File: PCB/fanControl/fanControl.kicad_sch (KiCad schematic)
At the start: 99 parts, among them J1 USB_B_Micro, J2 Barrel_Jack_Switch, J3 Conn_01x03, J4 Conn_01x06, J5 Conn_01x04, Q1 FDD4243, Q2 BSS84, Q3 BC547, Q4 BC847B, Q5 BC847B, Q6 BRCS4484, Q7 BC847B, Q8 BSS84, Q9 BC847B, U1 DS18B20, U2 CH340B, U3 LM2575BT-ADJ, U4 LM1117, U5 ESP-12E, Y1 12M

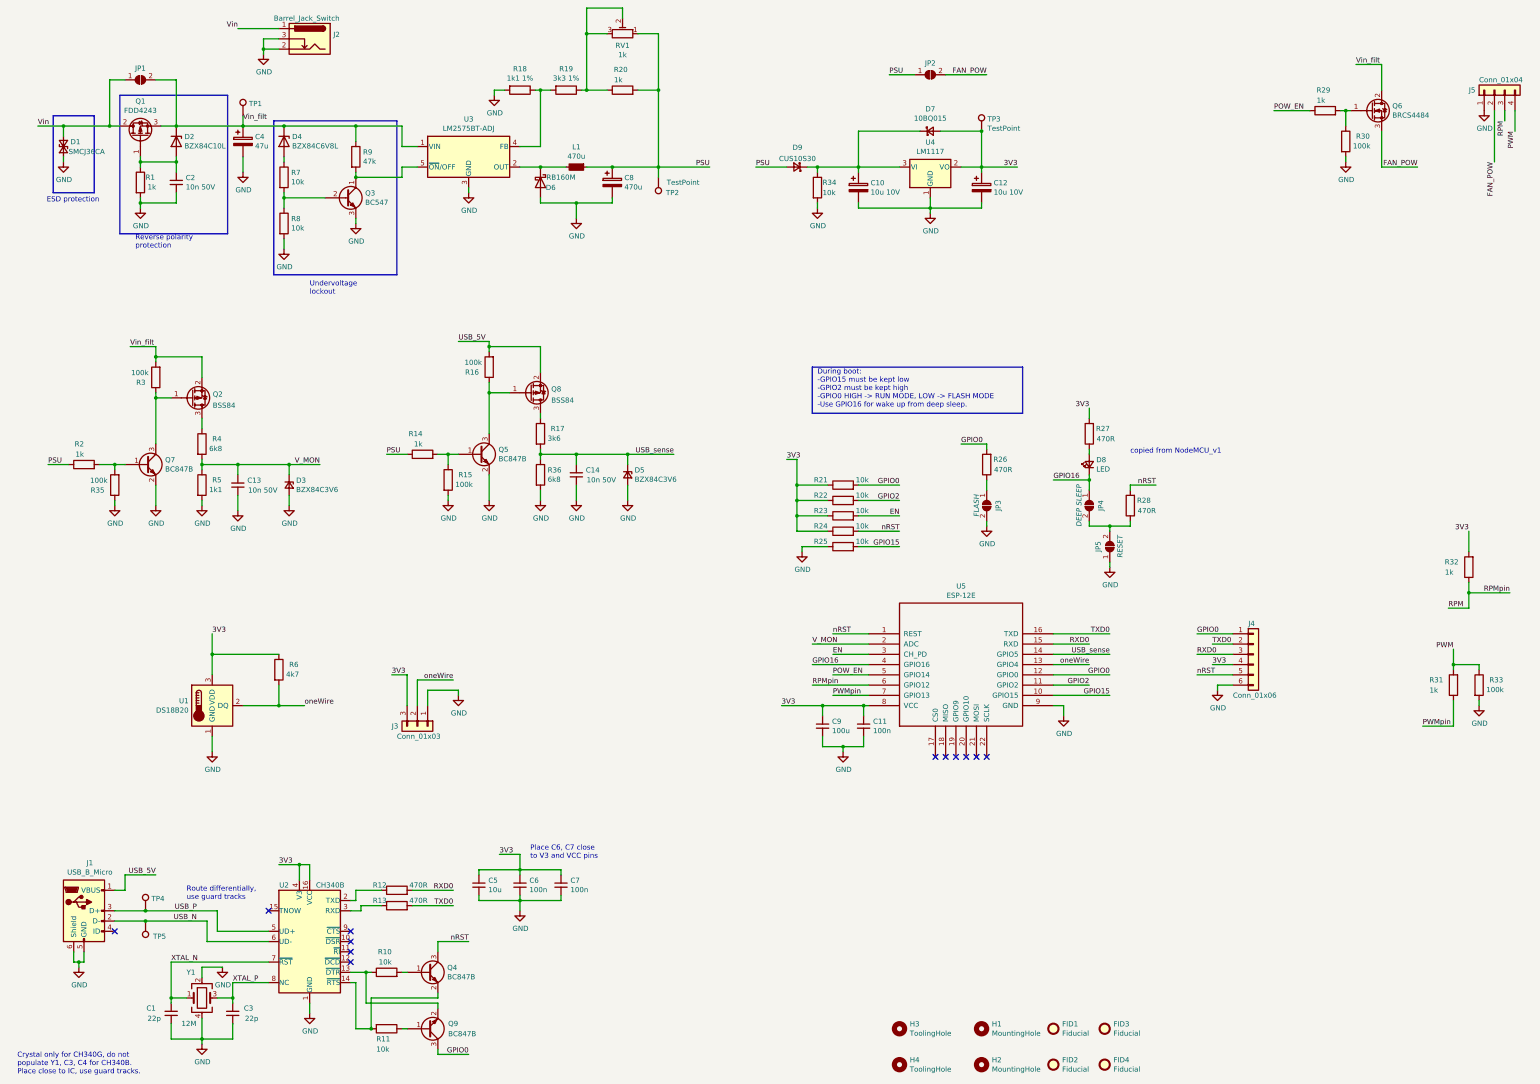
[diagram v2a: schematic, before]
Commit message: before optocouplers
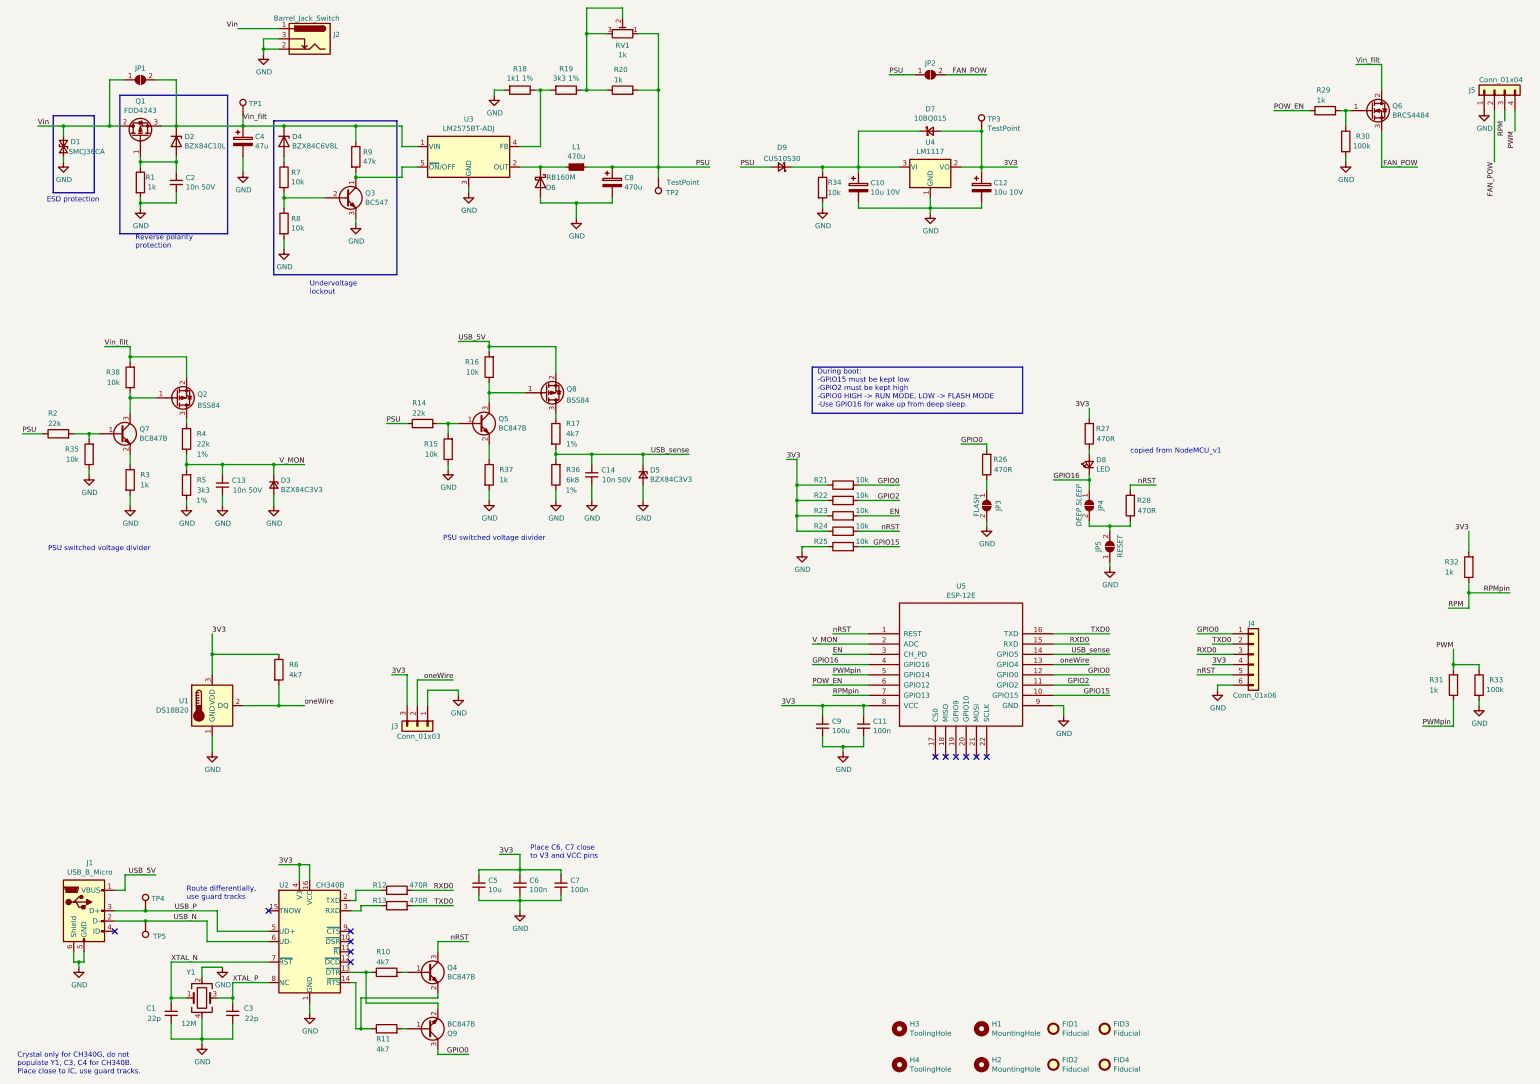
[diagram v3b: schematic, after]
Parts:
- added R37: 1k, agro-footprint:RES_0805, symbol Device:R
- added R38: 10k, agro-footprint:RES_0805, symbol Device:R
- D3, D5: value BZX84C3V6 -> BZX84C3V3; LCSC C94413 -> C82473; MPN BZX84C3V6LT1G -> BZX84C3V3LT1G
- D9, Q2, Q8: Supplier (none) -> LCSC
- R10, R11: value 10k -> 4k7; LCSC C100047 -> C60816; MPN RC0805JR-0710KL -> RC0805FR-074K7L; RMK (none) -> 1%
- R14, R2: value 1k -> 22k; LCSC C100046 -> C114565; MPN RC0805JR-071KL -> RC0805FR-0722KL; RMK (none) -> 1%
- R15, R16, R35: value 100k -> 10k; LCSC C100049 -> C100047; MPN RC0805JR-07100KL -> RC0805JR-0710KL
- R17: value 3k6 -> 4k7; LCSC C229201 -> C60816; MPN AC0805JR-073K6L -> RC0805FR-074K7L; RMK (none) -> 1%
- R3: value 100k -> 1k; LCSC C100049 -> C100046; MPN RC0805JR-07100KL -> RC0805JR-071KL
- R36: LCSC C137409 -> C114550; MPN RC0805JR-076K8L -> RC0805FR-076K8L; RMK (none) -> 1%
- R4: value 6k8 -> 22k; LCSC (none) -> C114565; MPN (none) -> RC0805FR-0722KL; RMK (none) -> 1%
- R5: value 1k1 -> 3k3; LCSC (none) -> C114531; MPN (none) -> RC0805FR-073K3L; RMK (none) -> 1%
- R6: LCSC C105427 -> C60816; MPN RC0805JR-074K7L -> RC0805FR-074K7L; RMK (none) -> 1%
- U5: footprint kicad-ESP8266:ESP-12E -> ESP8266:ESP-12E
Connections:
- net GND: now also R15.1, R3.2, R36.1, R5.1, R37.2; no longer Q5.2 (E), Q7.2 (E), R15.2, R36.2, R5.2
- net POW_EN: now also U5.6 (GPIO12); no longer U5.5 (GPIO14)
- net PWMpin: now also U5.5 (GPIO14); no longer U5.7 (GPIO13)
- net RPM: now also U5.7 (GPIO13); no longer U5.6 (GPIO12)
- net USB_sense: now also R36.2; no longer R36.1
- net V_MON: now also R5.2; no longer R5.1
- net Vin_filt: now also R38.2; no longer R3.2
- net at Q4.2 (E), U2.14 (~{RTS}): now also R11.1; no longer R11.2
- net at Q5.1 (B), R14.2: now also R15.2; no longer R15.1
- net at Q2.1 (G), Q7.3 (C): now also R38.1; no longer R3.1
- net at Q9.1 (B): now also R11.2; no longer R11.1
- new net: Q7.2 (E), R3.1
- new net: Q5.2 (E), R37.1
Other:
- note added: "PSU switched voltage divider"
- moved on the sheet: C13, C14, D3, D5, D9, Q2, Q5, Q7, Q8, R34

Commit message: RFQ2
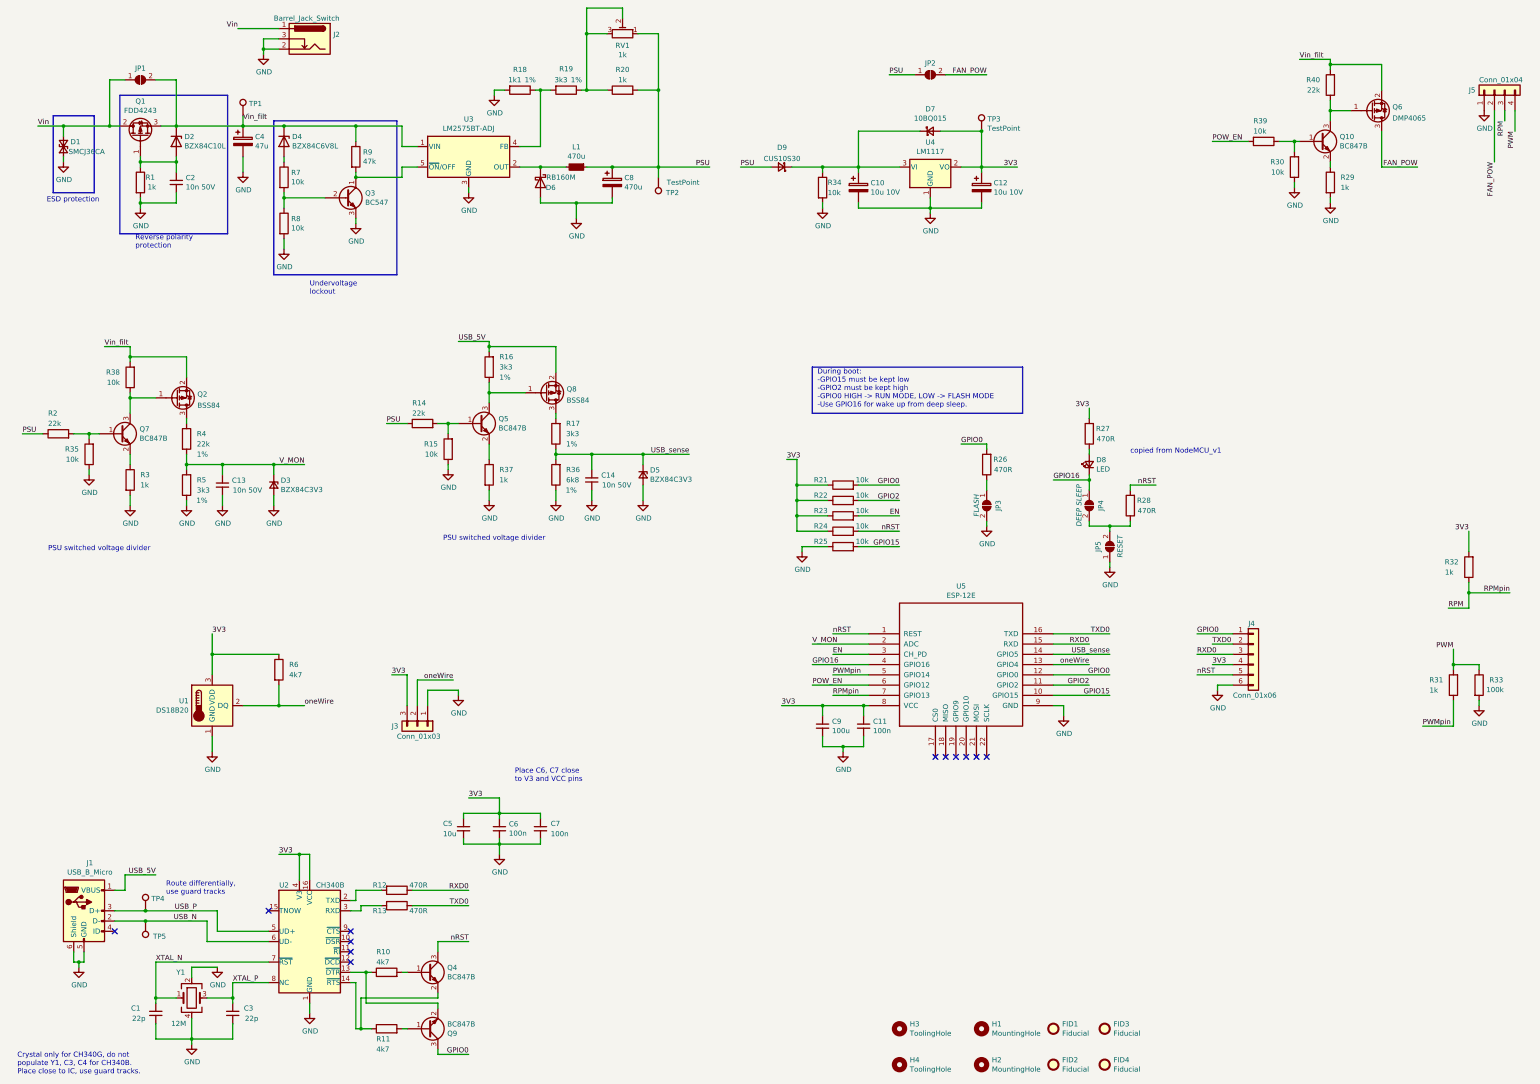
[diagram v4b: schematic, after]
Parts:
- removed Q6: BRCS4484, fanControl:BRCS4484, symbol Transistor_FET:IRF540N
- added Q10: BC847B, Package_TO_SOT_SMD:SOT-23, symbol Transistor_BJT:BC847
- added Q6: DMP4065, Package_TO_SOT_SMD:SOT-23, symbol Device:Q_PMOS_GSD
- added R39: 10k, agro-footprint:RES_0805, symbol Device:R
- added R40: 22k, agro-footprint:RES_0805, symbol Device:R
- R16: value 10k -> 3k3; LCSC C100047 -> C114531; MPN RC0805JR-0710KL -> RC0805FR-073K3L; RMK (none) -> 1%
- R17: value 4k7 -> 3k3; LCSC C60816 -> C114531; MPN RC0805FR-074K7L -> RC0805FR-073K3L
- R18: value 1k1 1% -> 1k1; RMK (none) -> 1%
- R19: value 3k3 1% -> 3k3; RMK (none) -> 1%
- R30: value 100k -> 10k; LCSC C100049 -> C100047; MPN RC0805JR-07100KL -> RC0805JR-0710KL
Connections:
- net FAN_POW: now also Q6.3 (D)
- net GND: now also R29.2, R30.1; no longer R30.2
- net POW_EN: now also R39.2; no longer R29.1
- net RXD0: now also R12.1; no longer R12.2
- net TXD0: now also R13.1; no longer R13.2
- net USB_sense: now also R17.1; no longer R17.2
- net Vin_filt: now also Q6.2 (S), R40.2
- net at U2.2 (TXD): now also R12.2; no longer R12.1
- net at U2.3 (RXD): now also R13.2; no longer R13.1
- net at Q8.3 (D): now also R17.2; no longer R17.1
- new net: Q10.3 (C), Q6.1 (G), R40.1
- new net: Q10.1 (B), R30.2, R39.1
- new net: Q10.2 (E), R29.1
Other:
- moved on the sheet: C1, C5, C6, C7, Y1

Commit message: ...
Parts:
- Q3: now in the parts list
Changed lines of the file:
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@@
   )
   (symbol (lib_id "Transistor_BJT:BC547") (at 96.52 64.77 0) (unit 1)
-    (in_bom no) (on_board yes)
+    (in_bom yes) (on_board yes)
     (property "Reference" "Q3" (id 0) (at 101.3714 63.6016 0)
       (effects (font (size 1.27 1.27)) (justify left))
@@
     (pin "2")
   )
+  (symbol (lib_id "Device:R") (at 132.08 133.35 0) (unit 1)
+    (in_bom yes) (on_board yes)
+    (property "Reference" "R37" (id 0) (at 134.62 132.08 0)
+      (effects (font (size 1.27 1.27)) (justify left))
+    )
+    (property "Value" "1k" (id 1) (at 134.62 134.62 0)
+      (effects (font (size 1.27 1.27)) (justify left))
+    )
+    (property "Footprint" "agro-footprint:RES_0805" (id 2) (at 130.302 133.35 90)
+      (effects (font (size 1.27 1.27)) hide)
+    )
+    (property "Datasheet" "https://datasheet.lcsc.com/lcsc/1810010217_YAGEO-RC0805JR-071KL_C100046.pdf" (id 3) (at 132.08 133.35 0)
+      (effects (font (size 1.27 1.27)) hide)
+    )
+    (property "Manufacturer" "Yageo" (id 4) (at 132.08 133.35 0)
+      (effects (font (size 1.27 1.27)) hide)
+    )
+    (property "MPN" "RC0805JR-071KL" (id 5) (at 132.08 133.35 0)
+      (effects (font (size 1.27 1.27)) hide)
+    )
+    (property "LCSC" "C100046" (id 6) (at 132.08 133.35 0)
+      (effects (font (size 1.27 1.27)) hide)
+    )
+    (property "Supplier" "LCSC" (id 7) (at 132.08 133.35 0)
+      (effects (font (size 1.27 1.27)) hide)
+    )
+    (pin "1")
+    (pin "2")
+  )
   (symbol (lib_id "power:GND") (at 121.92 132.08 0) (unit 1)
     (in_bom yes) (on_board yes)
@@
     (pin "2")
   )
-  (symbol (lib_id "Device:R") (at 132.08 133.35 0) (unit 1)
-    (in_bom yes) (on_board yes)
-    (property "Reference" "R37" (id 0) (at 134.62 132.08 0)
-      (effects (font (size 1.27 1.27)) (justify left))
-    )
-    (property "Value" "1k" (id 1) (at 134.62 134.62 0)
-      (effects (font (size 1.27 1.27)) (justify left))
-    )
-    (property "Footprint" "agro-footprint:RES_0805" (id 2) (at 130.302 133.35 90)
-      (effects (font (size 1.27 1.27)) hide)
-    )
-    (property "Datasheet" "https://datasheet.lcsc.com/lcsc/1810010217_YAGEO-RC0805JR-071KL_C100046.pdf" (id 3) (at 132.08 133.35 0)
-      (effects (font (size 1.27 1.27)) hide)
-    )
-    (property "Manufacturer" "Yageo" (id 4) (at 132.08 133.35 0)
-      (effects (font (size 1.27 1.27)) hide)
-    )
-    (property "MPN" "RC0805JR-071KL" (id 5) (at 132.08 133.35 0)
-      (effects (font (size 1.27 1.27)) hide)
-    )
-    (property "LCSC" "C100046" (id 6) (at 132.08 133.35 0)
-      (effects (font (size 1.27 1.27)) hide)
-    )
-    (property "Supplier" "LCSC" (id 7) (at 132.08 133.35 0)
-      (effects (font (size 1.27 1.27)) hide)
-    )
-    (pin "1")
-    (pin "2")
-  )
   (symbol (lib_id "Device:R") (at 219.71 139.7 90) (unit 1)
     (in_bom yes) (on_board yes)
@@
       (reference "R36") (unit 1) (value "6k8") (footprint "agro-footprint:RES_0805")
     )
-    (path "/9a7a10af-6813-48ac-8fc8-617b33ead1b5"
+    (path "/128a863a-a0d3-46d6-968e-217fb370d54c"
       (reference "R37") (unit 1) (value "1k") (footprint "agro-footprint:RES_0805")
     )
